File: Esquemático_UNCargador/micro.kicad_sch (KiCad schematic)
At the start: 15 parts, among them J2 Relay, J9 Conn_01x02_Pin, Q1 PN2222A, Q2 PN2222A

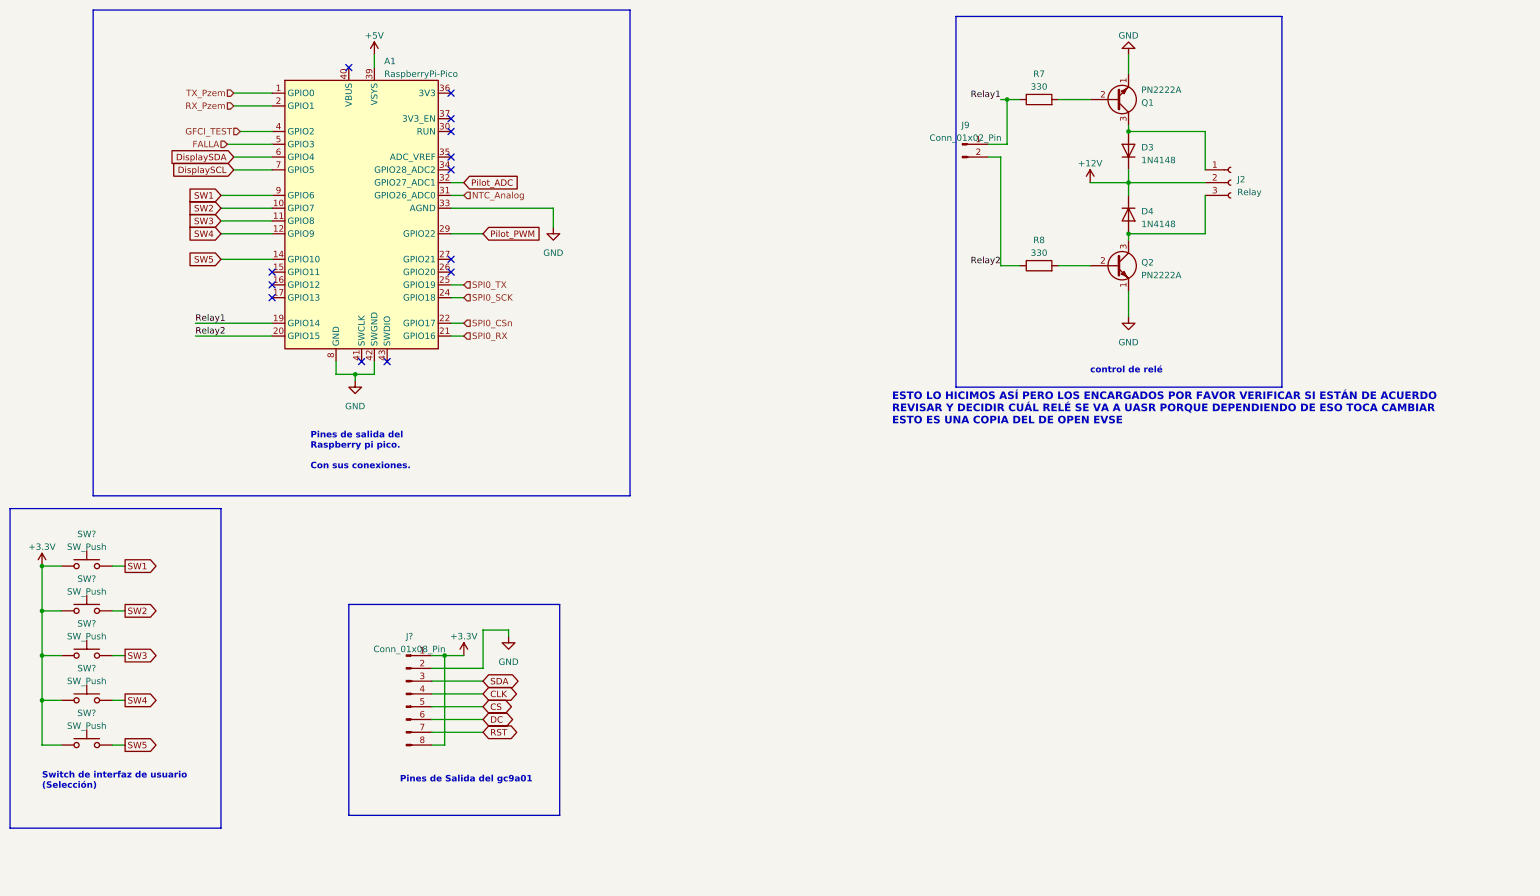
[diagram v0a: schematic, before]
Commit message: Modificación relays
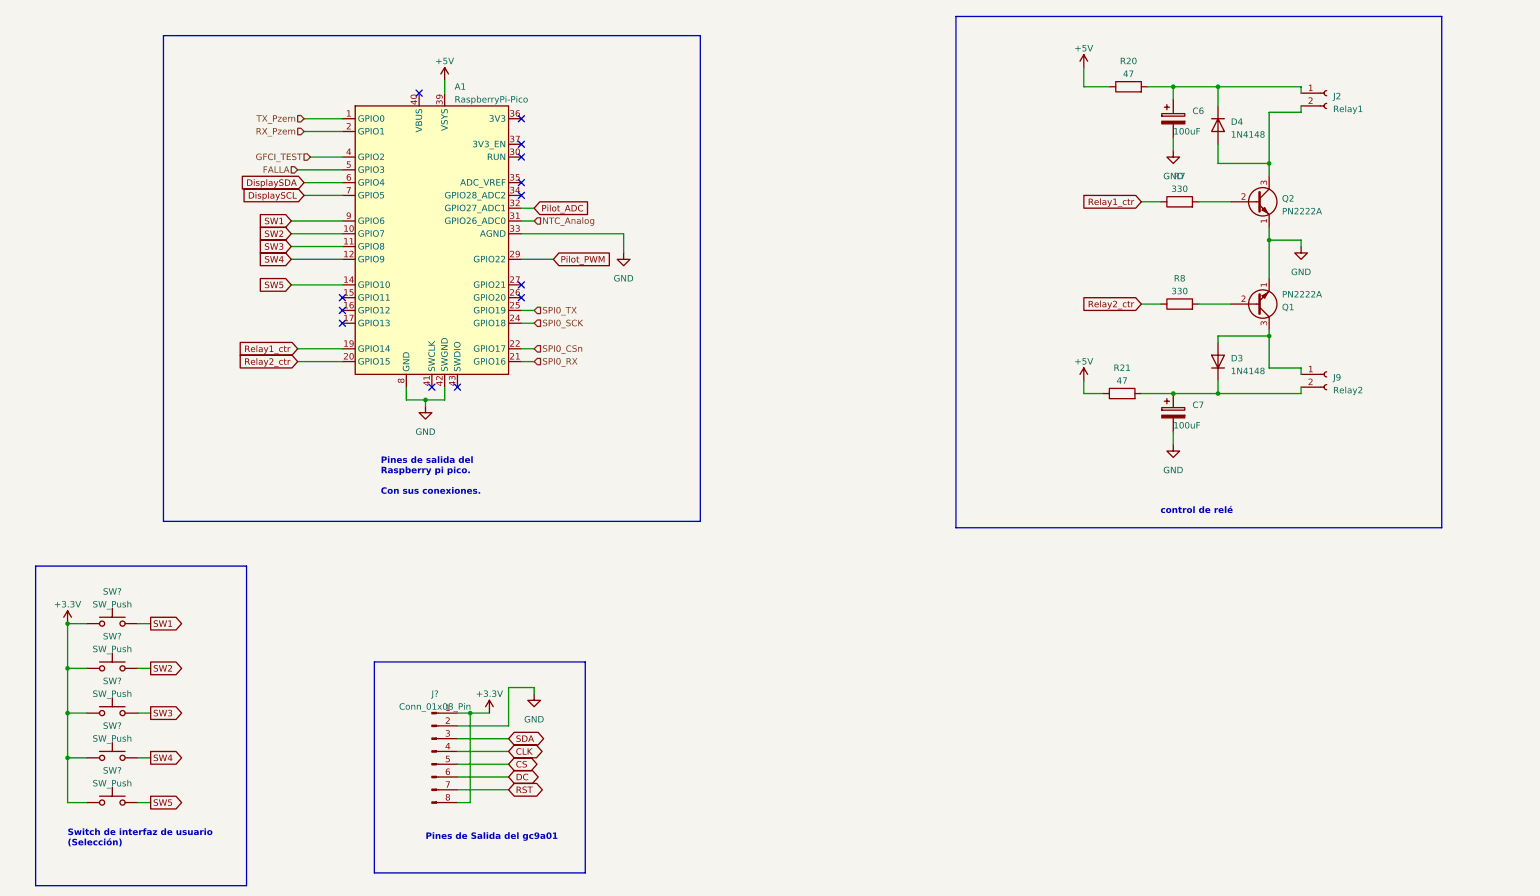
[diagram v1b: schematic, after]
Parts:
- removed J2: Relay, symbol Connector:Conn_01x03_Socket
- removed J9: Conn_01x02_Pin, symbol Connector:Conn_01x02_Pin
- added C6, C7: 100uF, Capacitor_THT:CP_Radial_D8.0mm_P3.50mm, symbol Device:C_Polarized
- added J2: Relay1, Connector_Molex:Molex_KK-254_AE-6410-02A_1x02_P2.54mm_Vertical, symbol Connector:Conn_01x02_Socket
- added J9: Relay2, Connector_Molex:Molex_KK-254_AE-6410-02A_1x02_P2.54mm_Vertical, symbol Connector:Conn_01x02_Socket
- added R20, R21: 47, Resistor_THT:R_Axial_DIN0207_L6.3mm_D2.5mm_P10.16mm_Horizontal, symbol Device:R
- R7, R8: footprint Resistor_THT:R_Axial_DIN0204_L3.6mm_D1.6mm_P5.08mm_Horizontal -> Resistor_THT:R_Axial_DIN0207_L6.3mm_D2.5mm_P10.16mm_Horizontal
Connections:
- net +5V: now also R20.1, R21.1
- net GND: now also C6.2, C7.2
- net at R8.2: now also Q1.2 (B); no longer Q2.2 (B)
- net at R7.2: now also Q2.2 (B); no longer Q1.2 (B)
- net at D4.2 (A), Q2.3 (C): now also J2.2 (Pin_2)
- net at D3.2 (A), Q1.3 (C): now also J9.1 (Pin_1)
- net +12V: no longer names the net of D3.1 (K)
- net +12V: now also C7.1, J9.2 (Pin_2), R21.2; no longer D4.1 (K)
- net Relay1 renamed Relay1_ctr
- net Relay2 renamed Relay2_ctr
- new net: C6.1, D4.1 (K), J2.1 (Pin_1), R20.2
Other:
- note removed: "ESTO LO HICIMOS ASÍ PERO LOS ENCARGADOS POR FAVOR VERIFICAR SI ESTÁN DE ACUERDO REVISAR Y DECIDIR CUÁL RELÉ SE VA A UASR PORQUE DEPENDIENDO DE ESO TOCA CAMBIAR ESTO ES UNA COPIA DEL DE OPEN EVSE"
- moved on the sheet: A1, J?, R7, R8, SW?

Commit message: Cambios de recomendaciones profesor
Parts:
- J?: footprint (none) -> Connector_PinHeader_2.54mm:PinHeader_1x08_P2.54mm_Vertical
- SW? (x5): footprint (none) -> Connector_PinHeader_2.54mm:PinHeader_1x02_P2.54mm_Vertical
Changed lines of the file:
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@@
       (effects (font (size 1.27 1.27)))
     )
-    (property "Footprint" "" (at 52.07 149.86 0)
+    (property "Footprint" "Connector_PinHeader_2.54mm:PinHeader_1x02_P2.54mm_Vertical" (at 52.07 149.86 0)
       (effects (font (size 1.27 1.27)) hide)
     )
@@
       (effects (font (size 1.27 1.27)))
     )
-    (property "Footprint" "" (at 52.07 167.64 0)
+    (property "Footprint" "Connector_PinHeader_2.54mm:PinHeader_1x02_P2.54mm_Vertical" (at 52.07 167.64 0)
       (effects (font (size 1.27 1.27)) hide)
     )
@@
       (effects (font (size 1.27 1.27)))
     )
-    (property "Footprint" "" (at 52.07 176.53 0)
+    (property "Footprint" "Connector_PinHeader_2.54mm:PinHeader_1x02_P2.54mm_Vertical" (at 52.07 176.53 0)
       (effects (font (size 1.27 1.27)) hide)
     )
@@
       (effects (font (size 1.27 1.27)))
     )
-    (property "Footprint" "" (at 52.07 158.75 0)
+    (property "Footprint" "Connector_PinHeader_2.54mm:PinHeader_1x02_P2.54mm_Vertical" (at 52.07 158.75 0)
       (effects (font (size 1.27 1.27)) hide)
     )
@@
       (effects (font (size 1.27 1.27)))
     )
-    (property "Footprint" "" (at 52.07 140.97 0)
+    (property "Footprint" "Connector_PinHeader_2.54mm:PinHeader_1x02_P2.54mm_Vertical" (at 52.07 140.97 0)
       (effects (font (size 1.27 1.27)) hide)
     )
@@
       (effects (font (size 1.27 1.27)))
     )
-    (property "Footprint" "" (at 115.57 171.45 0)
-      (effects (font (size 1.27 1.27)) hide)
-    )
+    (property "Footprint" "Connector_PinHeader_2.54mm:PinHeader_1x08_P2.54mm_Vertical" (at 115.57 171.45 0)
+      (effects (font (size 1.27 1.27)) hide)
+    )

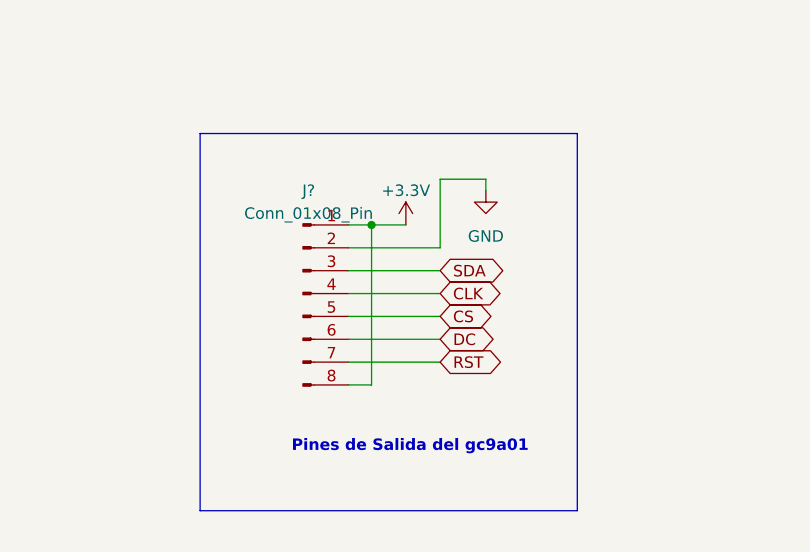
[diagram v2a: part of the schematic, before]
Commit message: version inicial layout PCB
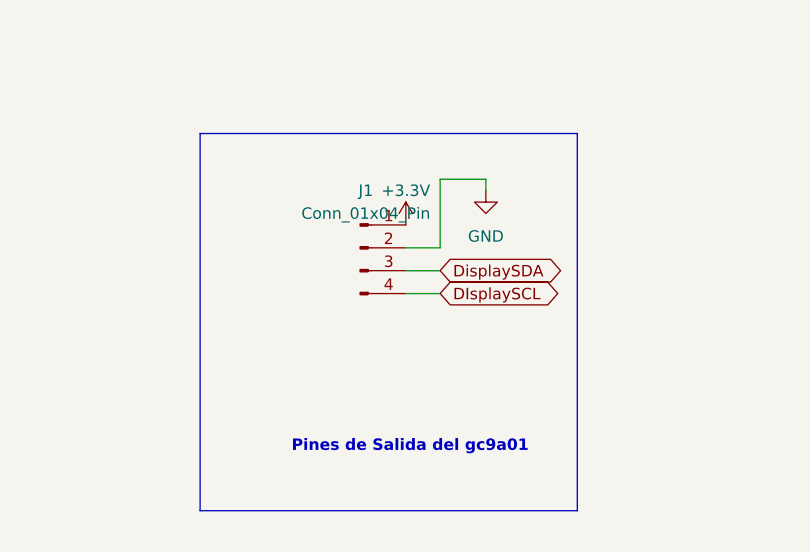
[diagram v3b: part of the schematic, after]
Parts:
- removed J?: Conn_01x08_Pin, Connector_PinHeader_2.54mm:PinHeader_1x08_P2.54mm_Vertical, symbol Connector:Conn_01x08_Pin
- added J1: Conn_01x04_Pin, Connector_PinHeader_2.54mm:PinHeader_1x04_P2.54mm_Vertical, symbol Connector:Conn_01x04_Pin
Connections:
- net +3.3V: now also J1.1 (Pin_1)
- net DisplaySDA: now also J1.3 (Pin_3)
- net GND: now also J1.2 (Pin_2)
- new net DIsplaySCL: J1.4 (Pin_4)
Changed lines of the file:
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@@
   (junction (at 271.78 39.37) (diameter 0) (color 0 0 0 0)
-  )
-  (junction (at 123.19 163.83) (diameter 0) (color 0 0 0 0)
   )
   (junction (at 262.89 39.37) (diameter 0) (color 0 0 0 0)
@@
     (stroke (width 0) (type default))
   )
+  (wire (pts (xy 127 166.37) (xy 130.81 166.37))
+    (stroke (width 0) (type default))
+  )
   (wire (pts (xy 87.63 66.04) (xy 97.79 66.04))
     (stroke (width 0) (type default))
   )
-  (wire (pts (xy 120.65 171.45) (xy 130.81 171.45))
-    (stroke (width 0) (type default))
-  )
   (wire (pts (xy 90.17 45.72) (xy 97.79 45.72))
     (stroke (width 0) (type default))
@@
     (stroke (width 0) (type default))
   )
-  (wire (pts (xy 123.19 163.83) (xy 127 163.83))
-    (stroke (width 0) (type default))
-  )
   (wire (pts (xy 91.44 53.34) (xy 97.79 53.34))
     (stroke (width 0) (type default))
@@
     (stroke (width 0) (type default))
   )
-  (wire (pts (xy 120.65 176.53) (xy 130.81 176.53))
-    (stroke (width 0) (type default))
-  )
   (wire (pts (xy 88.9 91.44) (xy 97.79 91.44))
     (stroke (width 0) (type default))
@@
     (stroke (width 0) (type default))
   )
-  (wire (pts (xy 120.65 166.37) (xy 130.81 166.37))
-    (stroke (width 0) (type default))
-  )
   (wire (pts (xy 271.78 39.37) (xy 271.78 43.18))
     (stroke (width 0) (type default))
@@
     (stroke (width 0) (type default))
   )
-  (wire (pts (xy 120.65 179.07) (xy 130.81 179.07))
-    (stroke (width 0) (type default))
-  )
   (wire (pts (xy 133.35 93.98) (xy 135.89 93.98))
     (stroke (width 0) (type default))
@@
     (stroke (width 0) (type default))
   )
-  (wire (pts (xy 120.65 181.61) (xy 123.19 181.61))
-    (stroke (width 0) (type default))
-  )
   (wire (pts (xy 288.29 99.06) (xy 288.29 100.33))
     (stroke (width 0) (type default))
   )
-  (wire (pts (xy 120.65 168.91) (xy 130.81 168.91))
-    (stroke (width 0) (type default))
-  )
   (wire (pts (xy 57.15 146.05) (xy 59.69 146.05))
     (stroke (width 0) (type default))
@@
     (stroke (width 0) (type default))
   )
-  (wire (pts (xy 120.65 173.99) (xy 130.81 173.99))
-    (stroke (width 0) (type default))
-  )
   (wire (pts (xy 90.17 58.42) (xy 97.79 58.42))
     (stroke (width 0) (type default))
@@
     (stroke (width 0) (type default))
   )
+  (wire (pts (xy 127 168.91) (xy 130.81 168.91))
+    (stroke (width 0) (type default))
+  )
   (wire (pts (xy 57.15 172.72) (xy 59.69 172.72))
     (stroke (width 0) (type default))
   )
-  (wire (pts (xy 123.19 181.61) (xy 123.19 163.83))
-    (stroke (width 0) (type default))
-  )
   (wire (pts (xy 288.29 39.37) (xy 288.29 40.64))
     (stroke (width 0) (type default))
@@
     (stroke (width 0) (type default))
   )
+  (wire (pts (xy 127 171.45) (xy 130.81 171.45))
+    (stroke (width 0) (type default))
+  )
   (wire (pts (xy 262.89 107.95) (xy 262.89 110.49))
     (stroke (width 0) (type default))
@@
   )
   (wire (pts (xy 267.97 82.55) (xy 274.32 82.55))
-    (stroke (width 0) (type default))
-  )
-  (wire (pts (xy 120.65 163.83) (xy 123.19 163.83))
     (stroke (width 0) (type default))
   )
@@
     (effects (font (size 1.27 1.27) (thickness 0.254) bold) (justify left bottom))
   )
-  (global_label "CS" (shape bidirectional) (at 130.81 173.99 0) (fields_autoplaced)
-    (effects (font (size 1.27 1.27)) (justify left))
-    (property "Intersheetrefs" "${INTERSHEET_REFS}" (at 137.3066 173.99 0)
-      (effects (font (size 1.27 1.27)) (justify left) hide)
-    )
-  )
-  (global_label "RST" (shape bidirectional) (at 130.81 179.07 0) (fields_autoplaced)
-    (effects (font (size 1.27 1.27)) (justify left))
-    (property "Intersheetrefs" "${INTERSHEET_REFS}" (at 138.2742 179.07 0)
-      (effects (font (size 1.27 1.27)) (justify left) hide)
-    )
-  )
   (global_label "SW2" (shape input) (at 87.63 68.58 180) (fields_autoplaced)
     (effects (font (size 1.27 1.27)) (justify right))
@@
     )
   )
-  (global_label "SDA" (shape bidirectional) (at 130.81 168.91 0) (fields_autoplaced)
-    (effects (font (size 1.27 1.27)) (justify left))
-    (property "Intersheetrefs" "${INTERSHEET_REFS}" (at 138.3952 168.91 0)
+  (global_label "DisplaySDA" (shape bidirectional) (at 130.81 168.91 0) (fields_autoplaced)
+    (effects (font (size 1.27 1.27)) (justify left))
+    (property "Intersheetrefs" "${INTERSHEET_REFS}" (at 145.2289 168.91 0)
       (effects (font (size 1.27 1.27)) (justify left) hide)
     )
@@
     )
   )
-  (global_label "CLK" (shape bidirectional) (at 130.81 171.45 0) (fields_autoplaced)
-    (effects (font (size 1.27 1.27)) (justify left))
-    (property "Intersheetrefs" "${INTERSHEET_REFS}" (at 138.3952 171.45 0)
+  (global_label "DIsplaySCL" (shape bidirectional) (at 130.81 171.45 0) (fields_autoplaced)
+    (effects (font (size 1.27 1.27)) (justify left))
+    (property "Intersheetrefs" "${INTERSHEET_REFS}" (at 145.1684 171.45 0)
       (effects (font (size 1.27 1.27)) (justify left) hide)
     )
@@
     (effects (font (size 1.27 1.27)) (justify left))
     (property "Intersheetrefs" "${INTERSHEET_REFS}" (at 66.4662 146.05 0)
-      (effects (font (size 1.27 1.27)) (justify left) hide)
-    )
-  )
-  (global_label "DC" (shape bidirectional) (at 130.81 176.53 0) (fields_autoplaced)
-    (effects (font (size 1.27 1.27)) (justify left))
-    (property "Intersheetrefs" "${INTERSHEET_REFS}" (at 137.3671 176.53 0)
       (effects (font (size 1.27 1.27)) (justify left) hide)
     )
@@
         (path "/f64e4c48-29c2-4644-b6e3-d55b9152fc29/27c27843-11c4-470f-a3f9-e81d775d20fc"
           (reference "SW5") (unit 1)
+        )
+      )
+    )
+  )
+  (symbol (lib_id "Connector:Conn_01x04_Pin") (at 121.92 166.37 0) (unit 1)
+    (in_bom yes) (on_board yes) (dnp no) (fields_autoplaced)
+    (property "Reference" "J1" (at 122.555 160.02 0)
+      (effects (font (size 1.27 1.27)))
+    )
+    (property "Value" "Conn_01x04_Pin" (at 122.555 162.56 0)
+      (effects (font (size 1.27 1.27)))
+    )
+    (property "Footprint" "Connector_PinHeader_2.54mm:PinHeader_1x04_P2.54mm_Vertical" (at 121.92 166.37 0)
+      (effects (font (size 1.27 1.27)) hide)
+    )
+    (property "Datasheet" "~" (at 121.92 166.37 0)
+      (effects (font (size 1.27 1.27)))
+    )
+    (pin "1")
+    (pin "2")
+    (pin "3")
+    (pin "4")
+    (instances
+      (project "CircuitoPotencia"
+        (path "/f64e4c48-29c2-4644-b6e3-d55b9152fc29/27c27843-11c4-470f-a3f9-e81d775d20fc"
+          (reference "J1") (unit 1)
         )
       )
@@
         )
       )
-    )
-  )
-  (symbol (lib_id "Connector:Conn_01x08_Pin") (at 115.57 171.45 0) (unit 1)
-    (in_bom yes) (on_board yes) (dnp no) (fields_autoplaced)
-    (property "Reference" "J?" (at 116.205 160.02 0)
-      (effects (font (size 1.27 1.27)))
-    )
-    (property "Value" "Conn_01x08_Pin" (at 116.205 162.56 0)
-      (effects (font (size 1.27 1.27)))
-    )
-    (property "Footprint" "Connector_PinHeader_2.54mm:PinHeader_1x08_P2.54mm_Vertical" (at 115.57 171.45 0)
-      (effects (font (size 1.27 1.27)) hide)
-    )
-    (property "Datasheet" "~" (at 115.57 171.45 0)
-      (effects (font (size 1.27 1.27)) hide)
-    )
-    (pin "1")
-    (pin "2")
-    (pin "3")
-    (pin "4")
-    (pin "5")
-    (pin "6")
-    (pin "7")
-    (pin "8")
-    (instances
-      (project "PreliminarPCB"
-        (path "/1ef7c57c-2fe6-466c-bcf5-d2e8b1f6c4da"
-          (reference "J?") (unit 1)
-        )
-      )
-      (project "CircuitoPotencia"
-        (path "/f64e4c48-29c2-4644-b6e3-d55b9152fc29/27c27843-11c4-470f-a3f9-e81d775d20fc"
-          (reference "J1") (unit 1)
-        )
-      )
